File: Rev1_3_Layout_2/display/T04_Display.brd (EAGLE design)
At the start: 63.5 x 53.5 mm, 57 parts, among them X2 22-23-2071

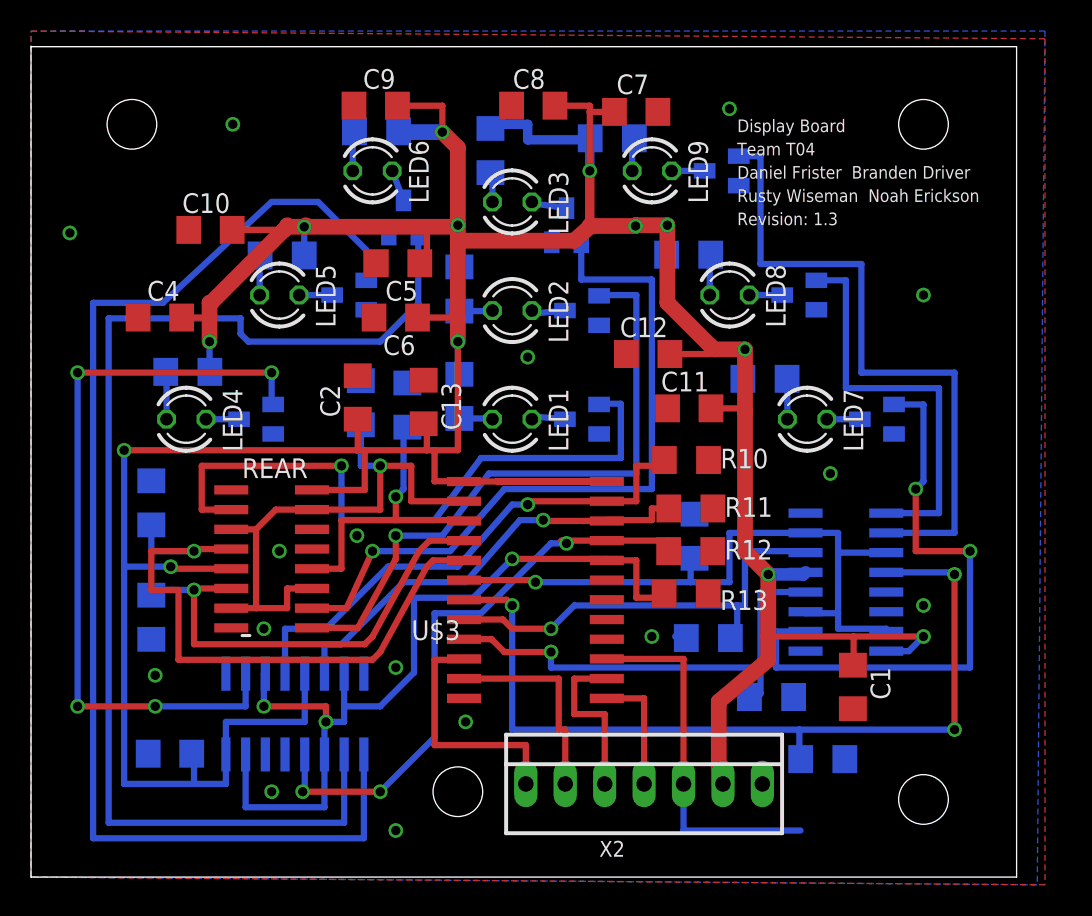
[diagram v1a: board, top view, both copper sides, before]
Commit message: Final Revision for display before submit.
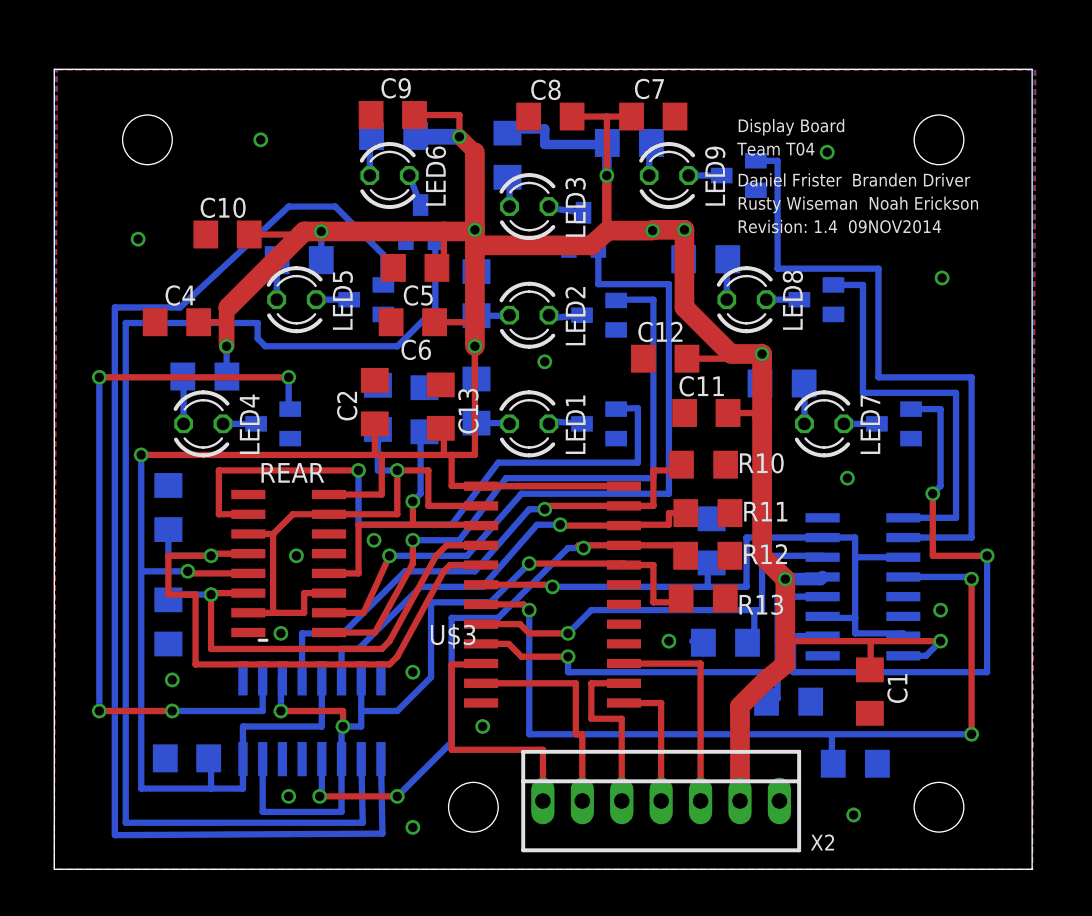
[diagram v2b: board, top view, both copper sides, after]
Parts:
- C13: value 0.1u -> 1u
- moved R19 2.12 mm to (51.6, 6.80)
- moved X2 1.56 mm to (39.1, 4.40)
- moved C8 1.30 mm to (32.0, 48.5)
- moved C9 1.25 mm to (21.8, 48.6)
- moved C12 1.14 mm to (39.4, 32.9)
- moved R2 1.14 mm to (42.0, 39.3)
- moved C11 1.14 mm to (42.0, 29.4)
- moved LED1 1.14 mm to (30.6, 28.7)
- moved LED7 1.14 mm to (49.6, 28.7)
- moved LEFT 1.14 mm to (16.6, 9.70)
- moved R1 1.14 mm to (46.9, 31.3)
- moved R10 1.14 mm to (41.8, 26.1)
- moved R11 1.14 mm to (42.1, 22.9)
- moved R12 1.14 mm to (42.1, 20.2)
- moved R13 1.14 mm to (41.8, 17.4)
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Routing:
- net N$7: track 23.5 -> 13.8 mm
- net RY: track 80.7 -> 79.1 mm
- net A0: track 15.8 -> 16.6 mm
- net A3: track 7.91 -> 8.71 mm
- net A2: track 10.8 -> 11.6 mm
- net A1: track 13.3 -> 14.1 mm
- net RG: track 49.1 -> 48.5 mm
- net GND: vias 16 -> 17
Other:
- board size 63.5 x 53.5 mm -> 63 x 51.5 mm
- board text added: "Revision: 1.4 09NOV2014"
- board text removed: "Revision: 1.3"
